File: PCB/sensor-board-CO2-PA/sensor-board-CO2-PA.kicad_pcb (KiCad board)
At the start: 2 copper layers, 23.6 x 23.5 mm, 8 parts, among them U1 MAGNETIC POGO CONN., U1 SCD40-D-R2, U2 MAGNETIC POGO CONN.

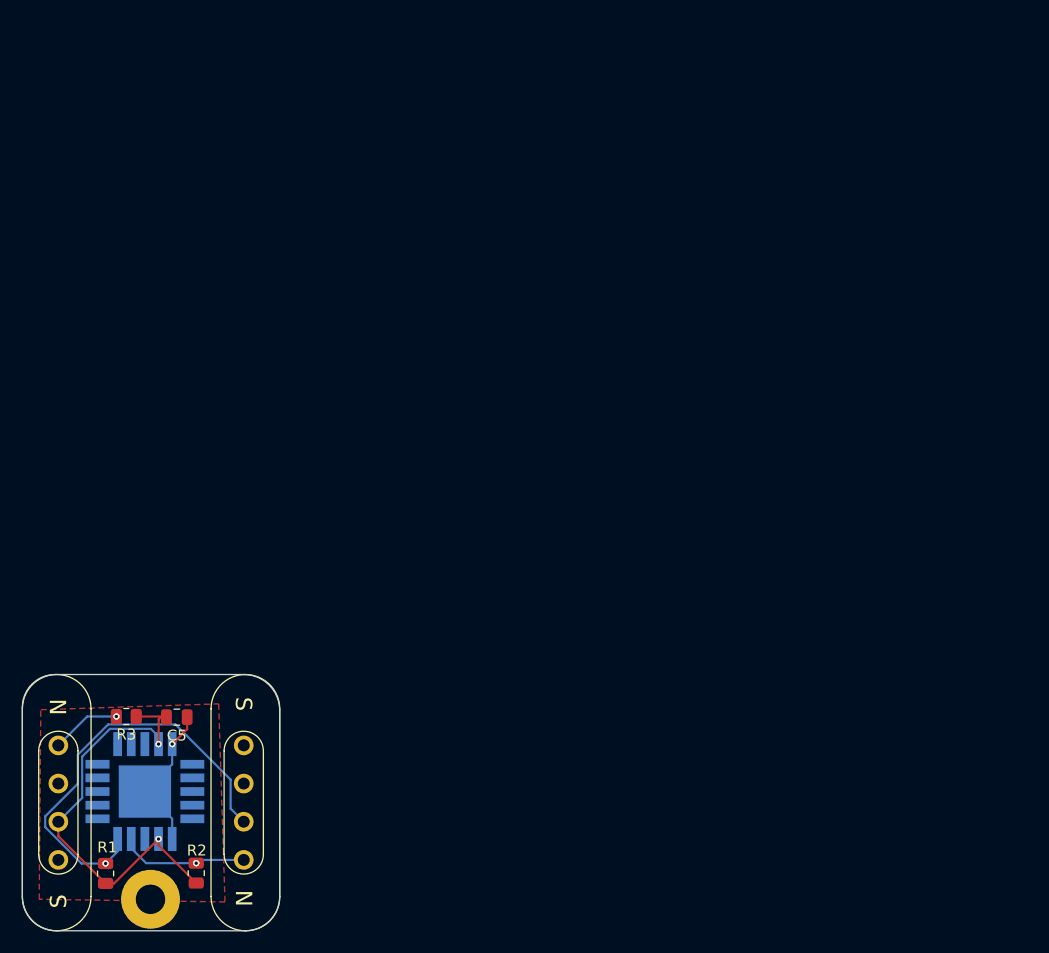
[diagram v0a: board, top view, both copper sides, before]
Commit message: made some changes
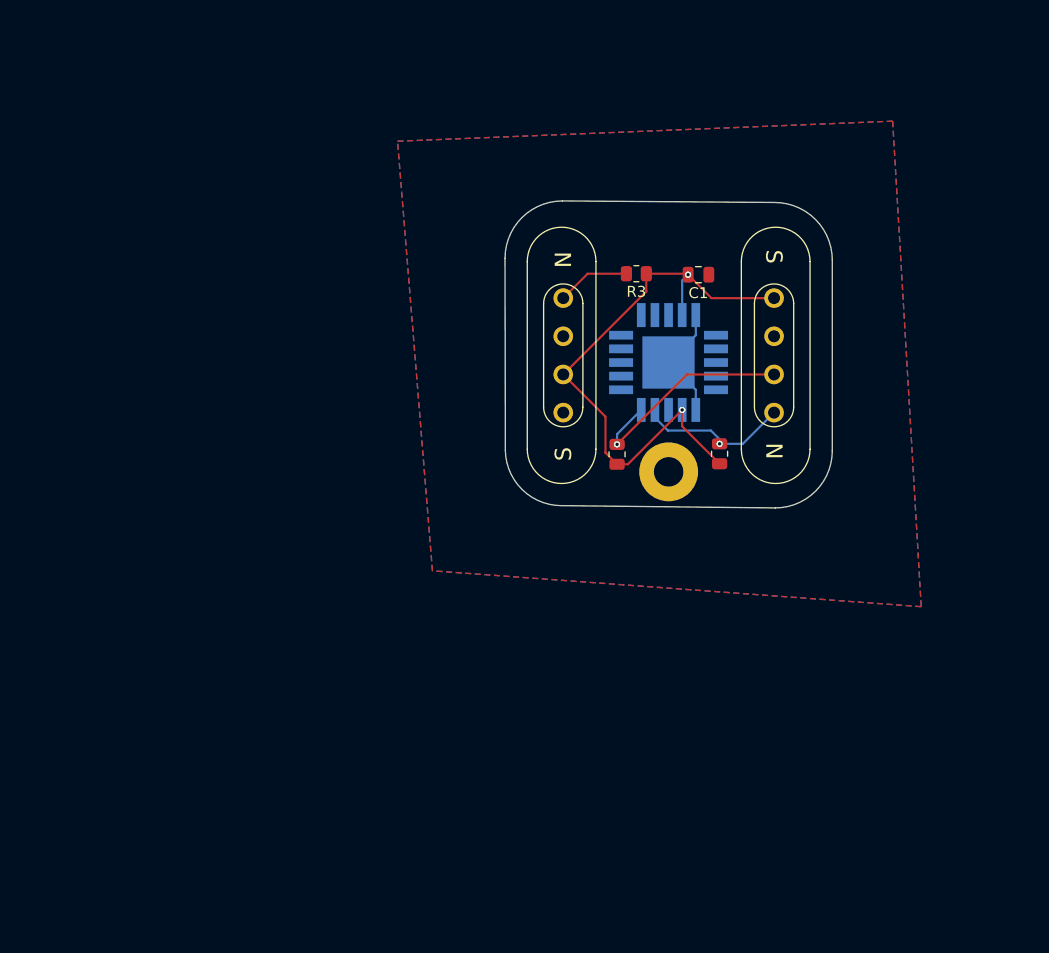
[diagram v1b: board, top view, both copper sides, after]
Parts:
- removed C5: 10microf, Capacitor_SMD:C_0805_2012Metric
- removed the U1 at (159.5, 106.0)
- removed the U1 at (150.5, 105.0)
- added C1: 10microf, Capacitor_SMD:C_0805_2012Metric, F.Cu at (201.2, 57.6)
- added G***: LOGO, LOGO, B.Cu at (188.2, 55.9)
- added G***: LOGO, LOGO, B.Cu at (209.4, 55.7)
- added U1: MAGNETIC POGO CONN., batteryholder:MAGNETIC POGO CONN., F.Cu at (208.2, 65.0)
- added U1: SCD40-D-R2, batteryholder:SCD40 footprint, B.Cu at (198.5, 65.7)
- moved R3 61.9 mm to (195.5, 57.5)
- moved U2 61.9 mm to (188.8, 65.0)
- moved H1 61.6 mm to (198.5, 75.7)
- moved R2 61.5 mm to (203.2, 74.0)
- moved R1 60.6 mm to (193.8, 74.1)
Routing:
- net /SDA: track 39.1 -> 21.1 mm
- net +3.3V: track 41.3 -> 54.1 mm
- net GND: track 13.8 -> 10.8 mm, vias 1 -> 0
- net /SCL: track 11.9 -> 14.1 mm
- net /ID: track 6.42 -> 6.72 mm, vias 1 -> 0
- added copper zone on B.Cu, net GND
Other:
- board size 23.6 x 23.5 mm -> 30 x 28.1 mm
- board text added: "BOREALIS"
- board text added: "CO2 Sensor"
- board text removed: "Borealis CO2 sensor"

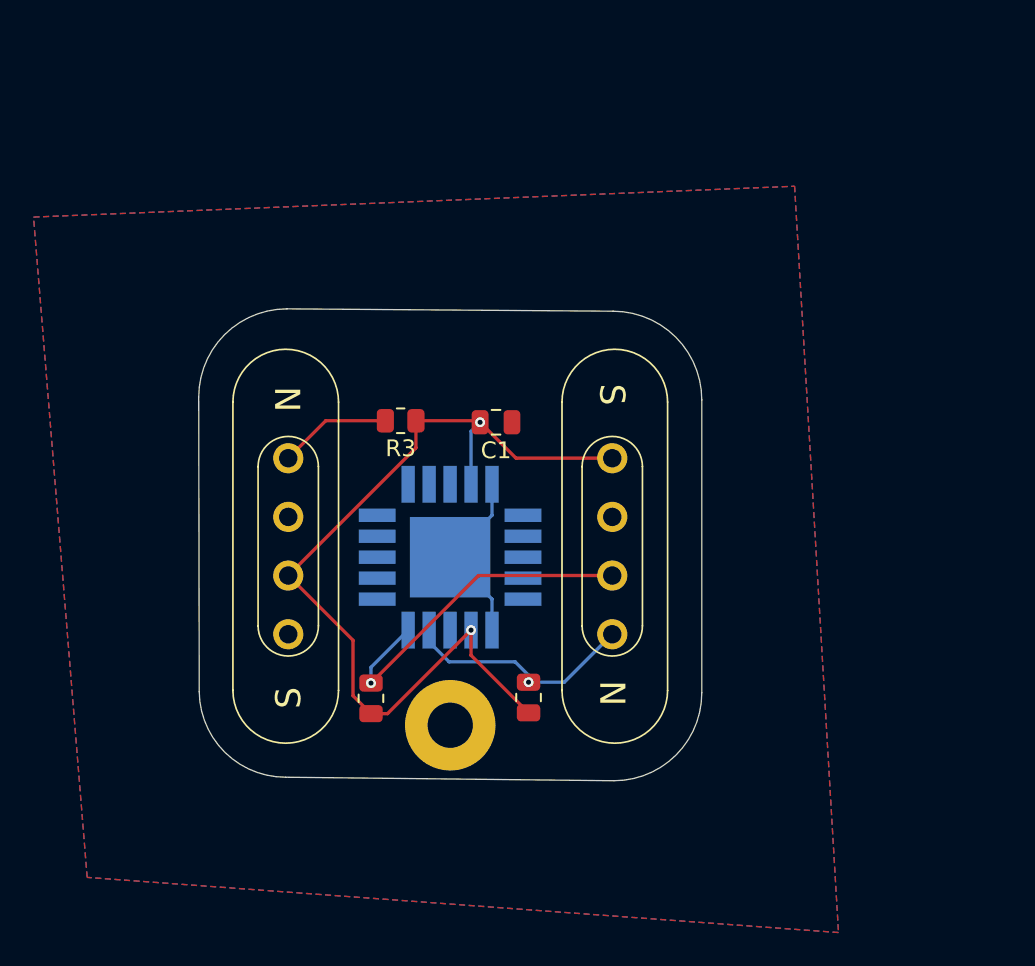
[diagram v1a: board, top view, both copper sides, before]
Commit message: Made some final checks and changes
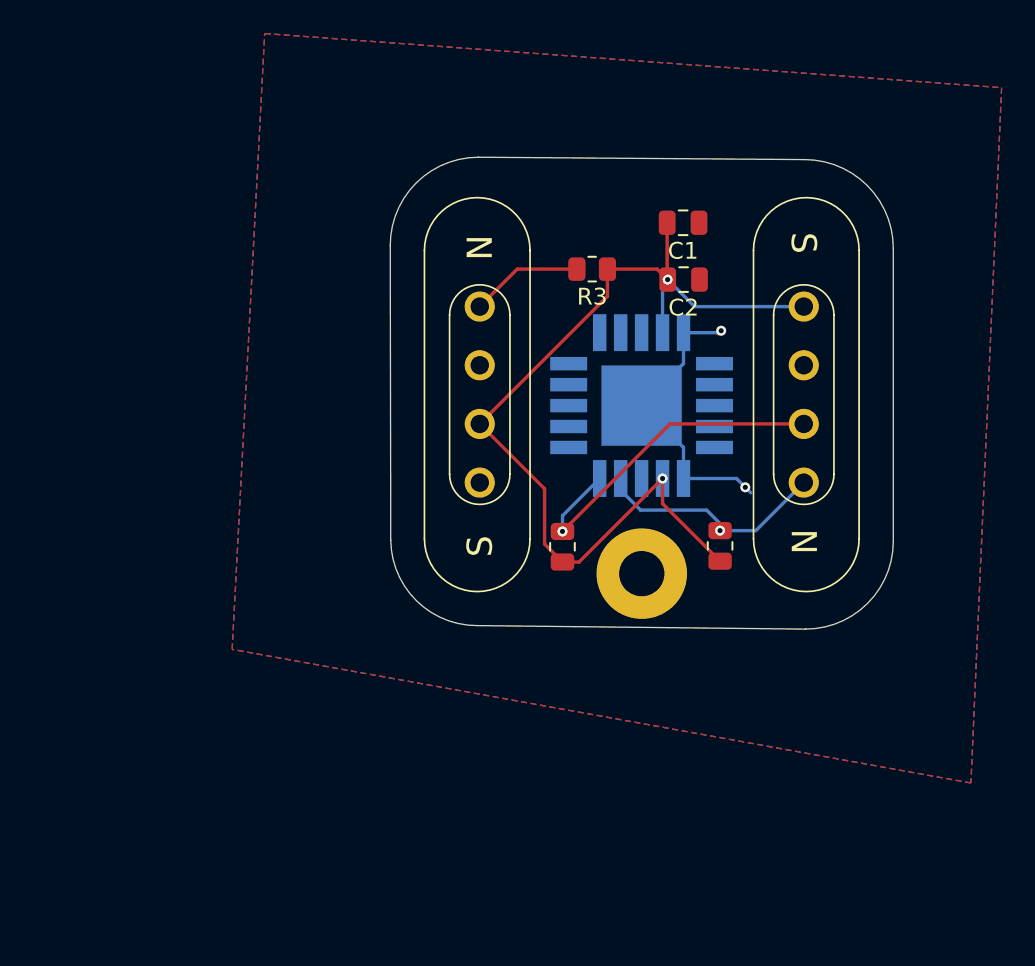
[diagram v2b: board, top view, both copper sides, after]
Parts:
- removed the G*** at (188.2, 55.9)
- removed the G*** at (209.4, 55.7)
- removed the U1 at (208.2, 65.0)
- removed the U1 at (198.5, 65.7)
- added C2: 0.1uf, Capacitor_SMD:C_0805_2012Metric, F.Cu at (212.4, 49.1)
- added G***: LOGO, LOGO, B.Cu at (220.9, 46.7)
- added G***: LOGO, LOGO, B.Cu at (199.7, 46.8)
- added U1: MAGNETIC POGO CONN., batteryholder:MAGNETIC POGO CONN., F.Cu at (219.6, 56.0)
- added U1: SCD40-D-R2, batteryholder:SCD40 footprint, B.Cu at (209.9, 56.6)
- moved C1 16.3 mm to (212.4, 45.7)
- moved R3 14.6 mm to (207.0, 48.5)
- moved U2 14.6 mm to (200.3, 56.0)
- moved H1 14.6 mm to (209.9, 66.6)
- moved R1 14.6 mm to (205.2, 65.0)
- moved R2 14.6 mm to (214.6, 65.0)
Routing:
- net GND: track 10.8 -> 17.7 mm, vias 0 -> 2
- net +3.3V: track 54.1 -> 57.0 mm
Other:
- board size 30 x 28.1 mm -> 30 x 28.2 mm
- board text added: "CO2 SENSOR"
- board text removed: "CO2 Sensor"
